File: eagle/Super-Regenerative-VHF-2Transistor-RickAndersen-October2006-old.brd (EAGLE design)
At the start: 45.7 x 30.5 mm, 25 parts, among them SW1 SL-SW-1P-2T-H, T1 2N3904, T2 2N3904

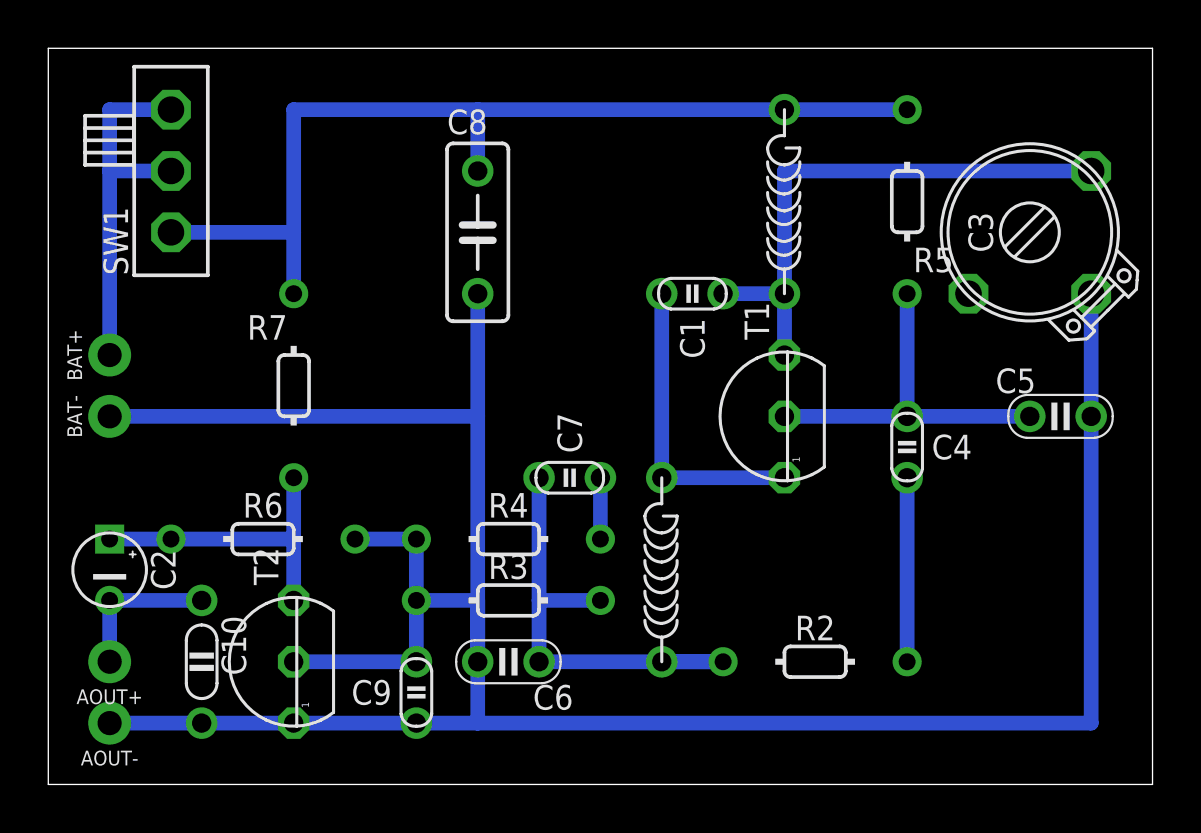
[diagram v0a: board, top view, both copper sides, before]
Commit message: ...
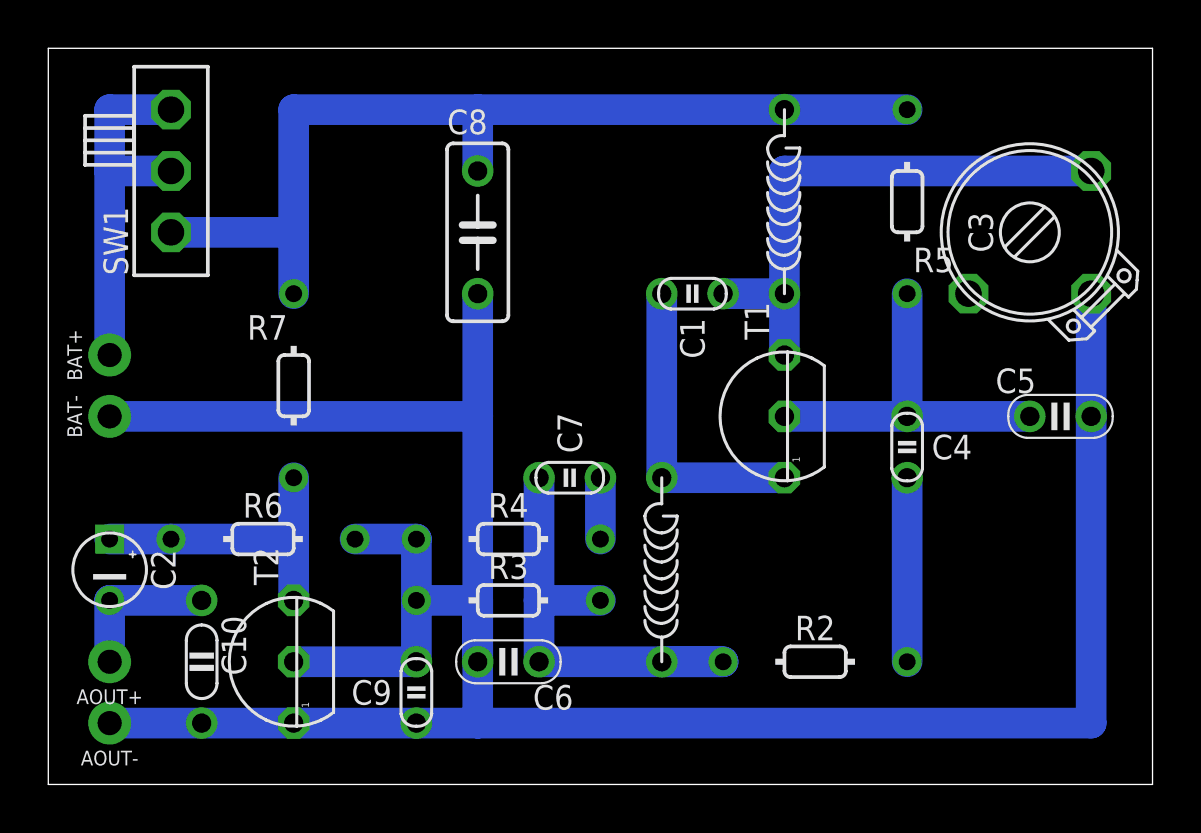
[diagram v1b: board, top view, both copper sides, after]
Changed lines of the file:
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@@
 <contactref element="L1" pad="1"/>
 <contactref element="C1" pad="2"/>
-<wire x1="27.94" y1="20.32" x2="30.48" y2="20.32" width="0.6096" layer="16"/>
+<wire x1="27.94" y1="20.32" x2="30.48" y2="20.32" width="1.27" layer="16"/>
 <contactref element="C3" pad="3"/>
-<wire x1="43.18" y1="25.4" x2="30.48" y2="25.4" width="0.6096" layer="16"/>
-<wire x1="30.48" y1="25.4" x2="30.48" y2="20.32" width="0.6096" layer="16"/>
+<wire x1="43.18" y1="25.4" x2="30.48" y2="25.4" width="1.27" layer="16"/>
+<wire x1="30.48" y1="25.4" x2="30.48" y2="20.32" width="1.27" layer="16"/>
 <contactref element="T1" pad="3"/>
-<wire x1="30.48" y1="17.78" x2="30.48" y2="20.32" width="0.6096" layer="16"/>
+<wire x1="30.48" y1="17.78" x2="30.48" y2="20.32" width="1.27" layer="16"/>
 </signal>
 <signal name="N$2">
 <contactref element="C1" pad="1"/>
 <contactref element="L2" pad="2"/>
-<wire x1="25.4" y1="20.32" x2="25.4" y2="12.7" width="0.6096" layer="16"/>
+<wire x1="25.4" y1="20.32" x2="25.4" y2="12.7" width="1.27" layer="16"/>
 <contactref element="T1" pad="1"/>
-<wire x1="30.48" y1="12.7" x2="25.4" y2="12.7" width="0.6096" layer="16"/>
+<wire x1="30.48" y1="12.7" x2="25.4" y2="12.7" width="1.27" layer="16"/>
 </signal>
 <signal name="N$3">
 <contactref element="L1" pad="2"/>
 <contactref element="C8" pad="1"/>
-<wire x1="30.48" y1="27.94" x2="35.56" y2="27.94" width="0.6096" layer="16"/>
-<wire x1="10.16" y1="27.94" x2="17.78" y2="27.94" width="0.6096" layer="16"/>
-<wire x1="30.48" y1="27.94" x2="17.78" y2="27.94" width="0.6096" layer="16"/>
-<wire x1="17.78" y1="27.94" x2="17.78" y2="25.4" width="0.6096" layer="16"/>
+<wire x1="30.48" y1="27.94" x2="35.56" y2="27.94" width="1.27" layer="16"/>
+<wire x1="10.16" y1="27.94" x2="17.78" y2="27.94" width="1.27" layer="16"/>
+<wire x1="30.48" y1="27.94" x2="17.78" y2="27.94" width="1.27" layer="16"/>
+<wire x1="17.78" y1="27.94" x2="17.78" y2="25.4" width="1.27" layer="16"/>
 <contactref element="R5" pad="1"/>
 <contactref element="R7" pad="2"/>
 <contactref element="SW1" pad="3"/>
-<wire x1="10.16" y1="22.86" x2="10.16" y2="27.94" width="0.6096" layer="16"/>
-<wire x1="10.16" y1="20.32" x2="10.16" y2="22.86" width="0.6096" layer="16"/>
-<wire x1="10.16" y1="22.86" x2="5.08" y2="22.86" width="0.6096" layer="16"/>
+<wire x1="10.16" y1="22.86" x2="10.16" y2="27.94" width="1.27" layer="16"/>
+<wire x1="10.16" y1="20.32" x2="10.16" y2="22.86" width="1.27" layer="16"/>
+<wire x1="10.16" y1="22.86" x2="5.08" y2="22.86" width="1.27" layer="16"/>
 <wire x1="5.08" y1="24.13" x2="5.08" y2="22.86" width="0" layer="19" extent="1-16"/>
 </signal>
@@
 <contactref element="C8" pad="2"/>
 <contactref element="BAT-" pad="1"/>
-<wire x1="43.18" y1="15.24" x2="43.18" y2="2.54" width="0.6096" layer="16"/>
-<wire x1="43.18" y1="2.54" x2="17.78" y2="2.54" width="0.6096" layer="16"/>
-<wire x1="17.78" y1="2.54" x2="17.78" y2="5.08" width="0.6096" layer="16"/>
-<wire x1="17.78" y1="15.24" x2="17.78" y2="5.08" width="0.6096" layer="16"/>
-<wire x1="2.54" y1="15.24" x2="17.78" y2="15.24" width="0.6096" layer="16"/>
-<wire x1="17.78" y1="15.24" x2="17.78" y2="20.32" width="0.6096" layer="16"/>
-<wire x1="17.78" y1="5.08" x2="17.78" y2="7.62" width="0.6096" layer="16"/>
-<wire x1="17.78" y1="7.62" x2="15.24" y2="7.62" width="0.6096" layer="16"/>
+<wire x1="43.18" y1="15.24" x2="43.18" y2="2.54" width="1.27" layer="16"/>
+<wire x1="43.18" y1="2.54" x2="17.78" y2="2.54" width="1.27" layer="16"/>
+<wire x1="17.78" y1="2.54" x2="17.78" y2="5.08" width="1.27" layer="16"/>
+<wire x1="17.78" y1="15.24" x2="17.78" y2="5.08" width="1.27" layer="16"/>
+<wire x1="2.54" y1="15.24" x2="17.78" y2="15.24" width="1.27" layer="16"/>
+<wire x1="17.78" y1="15.24" x2="17.78" y2="20.32" width="1.27" layer="16"/>
+<wire x1="17.78" y1="5.08" x2="17.78" y2="7.62" width="1.27" layer="16"/>
+<wire x1="17.78" y1="7.62" x2="15.24" y2="7.62" width="1.27" layer="16"/>
 <contactref element="C9" pad="2"/>
 <contactref element="C10" pad="2"/>
 <contactref element="AOUT-" pad="1"/>
-<wire x1="15.24" y1="2.54" x2="17.78" y2="2.54" width="0.6096" layer="16"/>
-<wire x1="43.18" y1="15.24" x2="43.18" y2="20.32" width="0.6096" layer="16"/>
+<wire x1="15.24" y1="2.54" x2="17.78" y2="2.54" width="1.27" layer="16"/>
+<wire x1="43.18" y1="15.24" x2="43.18" y2="20.32" width="1.27" layer="16"/>
 <contactref element="T2" pad="1"/>
-<wire x1="2.54" y1="2.54" x2="15.24" y2="2.54" width="0.6096" layer="16"/>
+<wire x1="2.54" y1="2.54" x2="15.24" y2="2.54" width="1.27" layer="16"/>
 <wire x1="6.35" y1="2.54" x2="2.54" y2="2.54" width="0" layer="19" extent="1-1"/>
 <wire x1="10.16" y1="2.54" x2="6.35" y2="2.54" width="0" layer="19" extent="1-1"/>
@@
 <contactref element="C5" pad="1"/>
 <contactref element="R5" pad="2"/>
-<wire x1="35.56" y1="15.24" x2="40.64" y2="15.24" width="0.6096" layer="16"/>
-<wire x1="35.56" y1="15.24" x2="35.56" y2="20.32" width="0.6096" layer="16"/>
+<wire x1="35.56" y1="15.24" x2="40.64" y2="15.24" width="1.27" layer="16"/>
+<wire x1="35.56" y1="15.24" x2="35.56" y2="20.32" width="1.27" layer="16"/>
 <contactref element="T1" pad="2"/>
-<wire x1="35.56" y1="15.24" x2="30.48" y2="15.24" width="0.6096" layer="16"/>
+<wire x1="35.56" y1="15.24" x2="30.48" y2="15.24" width="1.27" layer="16"/>
 </signal>
 <signal name="N$6">
@@
 <contactref element="L2" pad="1"/>
 <contactref element="C7" pad="2"/>
-<wire x1="20.32" y1="5.08" x2="20.32" y2="7.62" width="0.6096" layer="16"/>
-<wire x1="22.86" y1="7.62" x2="20.32" y2="7.62" width="0.6096" layer="16"/>
-<wire x1="20.32" y1="7.62" x2="20.32" y2="12.7" width="0.6096" layer="16"/>
-<wire x1="20.32" y1="5.08" x2="27.94" y2="5.08" width="0.6096" layer="16"/>
-<wire x1="25.4" y1="5.08" x2="27.94" y2="5.08" width="0.6096" layer="16"/>
+<wire x1="20.32" y1="5.08" x2="20.32" y2="7.62" width="1.27" layer="16"/>
+<wire x1="22.86" y1="7.62" x2="20.32" y2="7.62" width="1.27" layer="16"/>
+<wire x1="20.32" y1="7.62" x2="20.32" y2="12.7" width="1.27" layer="16"/>
+<wire x1="20.32" y1="5.08" x2="27.94" y2="5.08" width="1.27" layer="16"/>
+<wire x1="25.4" y1="5.08" x2="27.94" y2="5.08" width="1.27" layer="16"/>
 </signal>
 <signal name="N$7">
 <contactref element="R2" pad="1"/>
 <contactref element="C4" pad="1"/>
-<wire x1="35.56" y1="5.08" x2="35.56" y2="12.7" width="0.6096" layer="16"/>
+<wire x1="35.56" y1="5.08" x2="35.56" y2="12.7" width="1.27" layer="16"/>
 </signal>
 <signal name="N$8">
 <contactref element="R4" pad="1"/>
 <contactref element="C7" pad="1"/>
-<wire x1="22.86" y1="10.16" x2="22.86" y2="12.7" width="0.6096" layer="16"/>
+<wire x1="22.86" y1="10.16" x2="22.86" y2="12.7" width="1.27" layer="16"/>
 </signal>
 <signal name="N$9">
 <contactref element="BAT+" pad="1"/>
 <contactref element="SW1" pad="2"/>
-<wire x1="2.54" y1="17.78" x2="2.54" y2="25.4" width="0.6096" layer="16"/>
+<wire x1="2.54" y1="17.78" x2="2.54" y2="25.4" width="1.27" layer="16"/>
 <contactref element="SW1" pad="1"/>
-<wire x1="5.08" y1="25.4" x2="2.54" y2="25.4" width="0.6096" layer="16"/>
-<wire x1="2.54" y1="25.4" x2="2.54" y2="27.94" width="0.6096" layer="16"/>
-<wire x1="2.54" y1="27.94" x2="5.08" y2="27.94" width="0.6096" layer="16"/>
+<wire x1="5.08" y1="25.4" x2="2.54" y2="25.4" width="1.27" layer="16"/>
+<wire x1="2.54" y1="25.4" x2="2.54" y2="27.94" width="1.27" layer="16"/>
+<wire x1="2.54" y1="27.94" x2="5.08" y2="27.94" width="1.27" layer="16"/>
 </signal>
 <signal name="N$5">
@@
 <contactref element="R7" pad="1"/>
 <contactref element="C2" pad="+"/>
-<wire x1="10.16" y1="12.7" x2="10.16" y2="10.16" width="0.6096" layer="16"/>
-<wire x1="10.16" y1="10.16" x2="5.08" y2="10.16" width="0.6096" layer="16"/>
-<wire x1="2.54" y1="10.16" x2="5.08" y2="10.16" width="0.6096" layer="16"/>
+<wire x1="10.16" y1="12.7" x2="10.16" y2="10.16" width="1.27" layer="16"/>
+<wire x1="10.16" y1="10.16" x2="5.08" y2="10.16" width="1.27" layer="16"/>
+<wire x1="2.54" y1="10.16" x2="5.08" y2="10.16" width="1.27" layer="16"/>
 <contactref element="T2" pad="3"/>
-<wire x1="10.16" y1="7.62" x2="10.16" y2="10.16" width="0.6096" layer="16"/>
+<wire x1="10.16" y1="7.62" x2="10.16" y2="10.16" width="1.27" layer="16"/>
 </signal>
 <signal name="N$10">
@@
 <contactref element="R4" pad="2"/>
 <contactref element="C9" pad="1"/>
-<wire x1="15.24" y1="10.16" x2="12.7" y2="10.16" width="0.6096" layer="16"/>
+<wire x1="15.24" y1="10.16" x2="12.7" y2="10.16" width="1.27" layer="16"/>
 <contactref element="T2" pad="2"/>
-<wire x1="15.24" y1="5.08" x2="10.16" y2="5.08" width="0.6096" layer="16"/>
-<wire x1="15.24" y1="5.08" x2="15.24" y2="10.16" width="0.6096" layer="16"/>
+<wire x1="15.24" y1="5.08" x2="10.16" y2="5.08" width="1.27" layer="16"/>
+<wire x1="15.24" y1="5.08" x2="15.24" y2="10.16" width="1.27" layer="16"/>
 </signal>
 <signal name="N$11">
@@
 <contactref element="C10" pad="1"/>
 <contactref element="AOUT+" pad="1"/>
-<wire x1="2.54" y1="7.62" x2="6.35" y2="7.62" width="0.6096" layer="16"/>
-<wire x1="2.54" y1="5.08" x2="2.54" y2="7.62" width="0.6096" layer="16"/>
+<wire x1="2.54" y1="7.62" x2="6.35" y2="7.62" width="1.27" layer="16"/>
+<wire x1="2.54" y1="5.08" x2="2.54" y2="7.62" width="1.27" layer="16"/>
 </signal>
 </signals>
